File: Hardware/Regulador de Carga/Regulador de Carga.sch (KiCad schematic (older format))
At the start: 16 parts

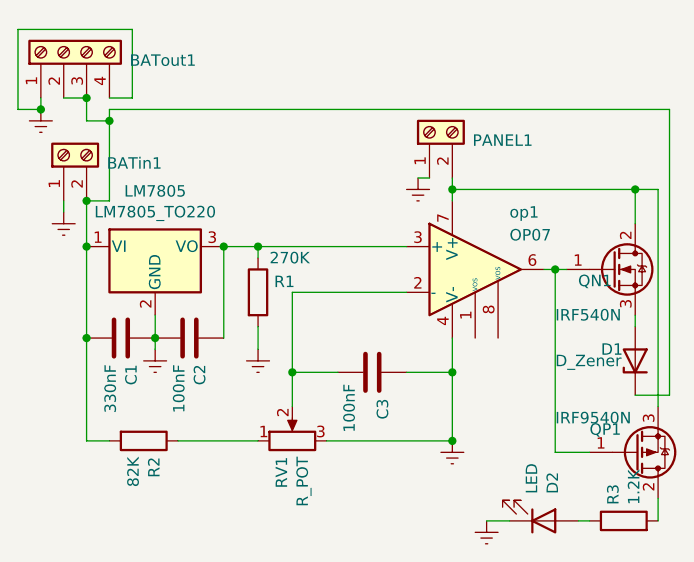
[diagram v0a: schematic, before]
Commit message: Actualizacion de placas
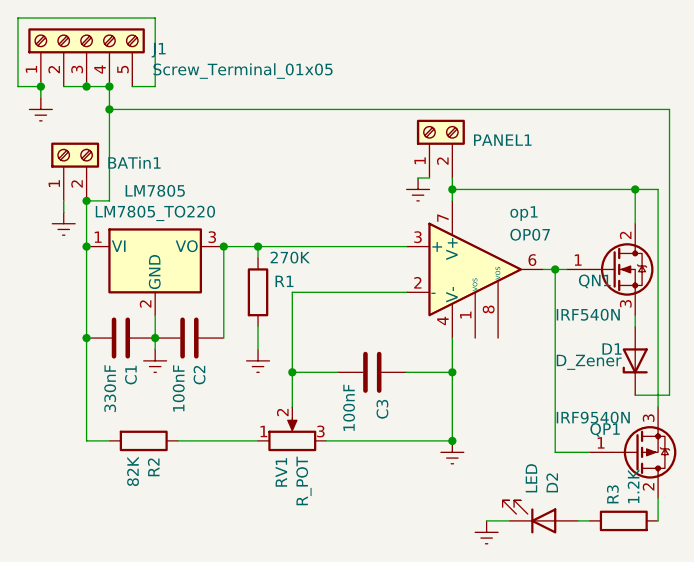
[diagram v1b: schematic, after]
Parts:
- removed BATout1: Screw_Terminal_01x04, TerminalBlock:TerminalBlock_bornier-4_P5.08mm, symbol Connector:Screw_Terminal_01x04
- added J1: Screw_Terminal_01x05, TerminalBlock:TerminalBlock_bornier-5_P5.08mm, symbol Connector:Screw_Terminal_01x05
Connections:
- net Earth: now also J1.1 (Pin_1), J1.5 (Pin_5)
- net at BATin1.2 (Pin_2), C1.2, D1.1 (K)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: now also J1.2 (Pin_2), J1.3 (Pin_3), J1.4 (Pin_4)
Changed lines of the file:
@@
 $EndDescr
-$Comp
-L Connector:Screw_Terminal_01x04 BATout1
-U 1 1 5E9E2845
-P 4400 1900
-F 0 "BATout1" V 4364 1612 50  0000 R CNN
-F 1 "Screw_Terminal_01x04" V 4273 1612 50  0001 R CNN
-F 2 "TerminalBlock:TerminalBlock_bornier-4_P5.08mm" H 4400 1900 50  0001 C CNN
-F 3 "~" H 4400 1900 50  0001 C CNN
-	1    4400 1900
-	0    -1   -1   0
-$EndComp
-Wire Wire Line
-	4400 2100 4500 2100
 $Comp
 L power:Earth #PWR0101
 U 1 1 5E9E4EF0
-P 4300 2150
-F 0 "#PWR0101" H 4300 1900 50  0001 C CNN
-F 1 "Earth" H 4300 2000 50  0001 C CNN
-F 2 "" H 4300 2150 50  0001 C CNN
-F 3 "~" H 4300 2150 50  0001 C CNN
-	1    4300 2150
-	1    0    0    -1
-$EndComp
-Wire Wire Line
-	4300 2100 4300 2150
-Wire Wire Line
-	4600 2100 4700 2100
-Wire Wire Line
-	4700 2100 4700 1800
-Wire Wire Line
-	4700 1800 4200 1800
-Wire Wire Line
-	4200 1800 4200 2150
-Wire Wire Line
-	4200 2150 4300 2150
-Connection ~ 4300 2150
+P 4300 2100
+F 0 "#PWR0101" H 4300 1850 50  0001 C CNN
+F 1 "Earth" H 4300 1950 50  0001 C CNN
+F 2 "" H 4300 2100 50  0001 C CNN
+F 3 "~" H 4300 2100 50  0001 C CNN
+	1    4300 2100
+	1    0    0    -1
+$EndComp
 $Comp
 L Connector:Screw_Terminal_01x02 BATin1
@@
 $EndComp
 Wire Wire Line
-	4500 2100 4500 2200
-Wire Wire Line
-	4500 2200 4600 2200
-Wire Wire Line
-	4600 2200 4600 2550
-Wire Wire Line
 	4600 2550 4500 2550
-Connection ~ 4500 2100
 Connection ~ 4500 2550
-Wire Wire Line
-	4600 2150 4600 2200
-Connection ~ 4600 2200
 $Comp
 L Device:R R3
@@
 Wire Wire Line
 	4500 3600 4600 3600
+Wire Wire Line
+	4600 2150 4600 2550
+$Comp
+L Connector:Screw_Terminal_01x05 J1
+U 1 1 5EFA25E1
+P 4500 1850
+F 0 "J1" V 4464 1562 50  0000 R CNN
+F 1 "Screw_Terminal_01x05" V 4373 1562 50  0000 R CNN
+F 2 "TerminalBlock:TerminalBlock_bornier-5_P5.08mm" H 4500 1850 50  0001 C CNN
+F 3 "~" H 4500 1850 50  0001 C CNN
+	1    4500 1850
+	0    -1   -1   0
+$EndComp
+Wire Wire Line
+	4600 2050 4500 2050
+Wire Wire Line
+	4400 2050 4500 2050
+Connection ~ 4500 2050
+Wire Wire Line
+	4600 2050 4600 2150
+Connection ~ 4600 2050
+Connection ~ 4600 2150
+Wire Wire Line
+	4700 2050 4800 2050
+Wire Wire Line
+	4800 2050 4800 1750
+Wire Wire Line
+	4800 1750 4200 1750
+Wire Wire Line
+	4200 1750 4200 2050
+Wire Wire Line
+	4200 2050 4300 2050
+Wire Wire Line
+	4300 2050 4300 2100
+Connection ~ 4300 2050
 $EndSCHEMATC

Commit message: Preparar para impresion
Prepare todas las placas para imprimirlas
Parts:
- RV1: footprint Potentiometer_THT:Potentiometer_ACP_CA14-H5_Horizontal -> Potentiometer_THT:Potentiometer_Bourns_3296W_Vertical
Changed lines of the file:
@@
 F 0 "RV1" H 5331 3646 50  0000 R CNN
 F 1 "R_POT" H 5331 3555 50  0000 R CNN
-F 2 "Potentiometer_THT:Potentiometer_ACP_CA14-H5_Horizontal" H 5400 3600 50  0001 C CNN
+F 2 "Potentiometer_THT:Potentiometer_Bourns_3296W_Vertical" H 5400 3600 50  0001 C CNN
 F 3 "~" H 5400 3600 50  0001 C CNN
 	1    5400 3600
